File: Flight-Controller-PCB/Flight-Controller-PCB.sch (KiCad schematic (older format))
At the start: 24 parts, among them J1 Power_In, J2 ESC_1, J3 ESC_2, J4 ESC_3, J5 ESC_4, J6 Receiver, J7 Aux, U1 MCP6001U

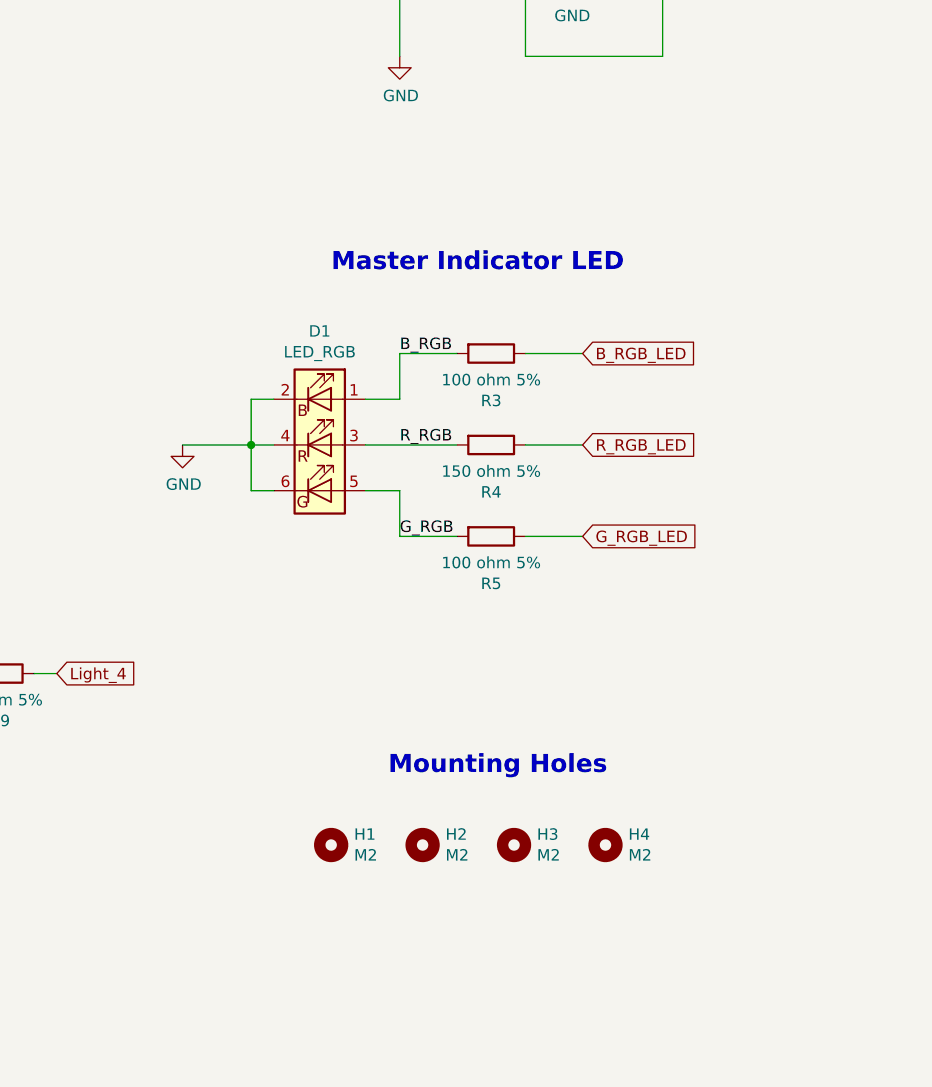
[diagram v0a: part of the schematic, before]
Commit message: Push before branch switch
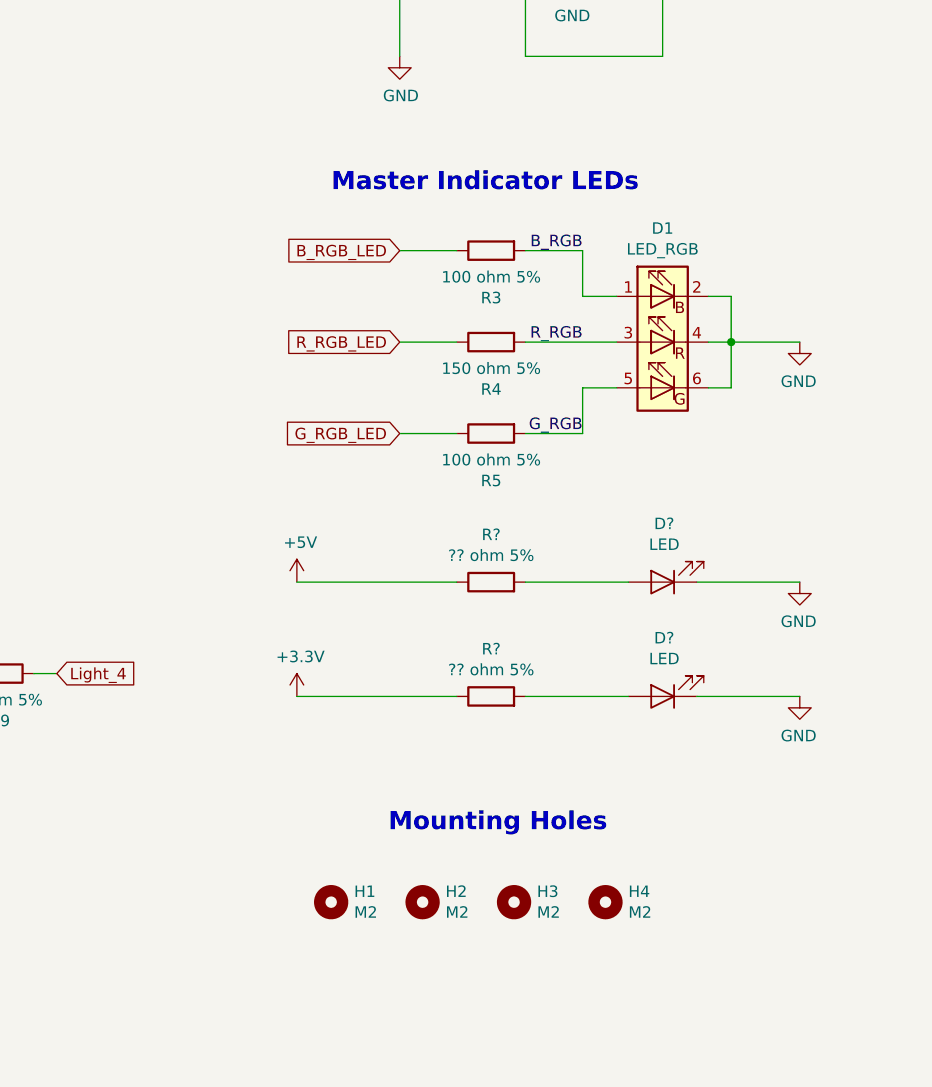
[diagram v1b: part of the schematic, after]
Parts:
- added D? (x2): LED, LED_SMD:LED_0603_1608Metric_Pad1.05x0.95mm_HandSolder, symbol Device:LED
- added R? (x2): ?? ohm 5%, Resistor_SMD:R_0603_1608Metric_Pad1.05x0.95mm_HandSolder, symbol Device:R
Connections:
- net +5V: now also R?.1
- net GND: now also D?.1 (K), D?.1 (K)
- new net: D?.2 (A), R?.2 (x2)
- new net +3V3: R?.1
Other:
- note added: "Master Indicator LEDs"
- note removed: "Master Indicator LED"
- moved on the sheet: D1, H1, H2, H3, H4, R3, R4, R5
